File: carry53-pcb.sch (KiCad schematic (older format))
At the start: 127 parts, among them J1 Conn_01x02, J2 Conn_01x03, SW1 TS-1187A-B-A-B, SW2 TS-1187A-B-A-B, U1 STM32F072CBT6, U2 XC6206P332MR

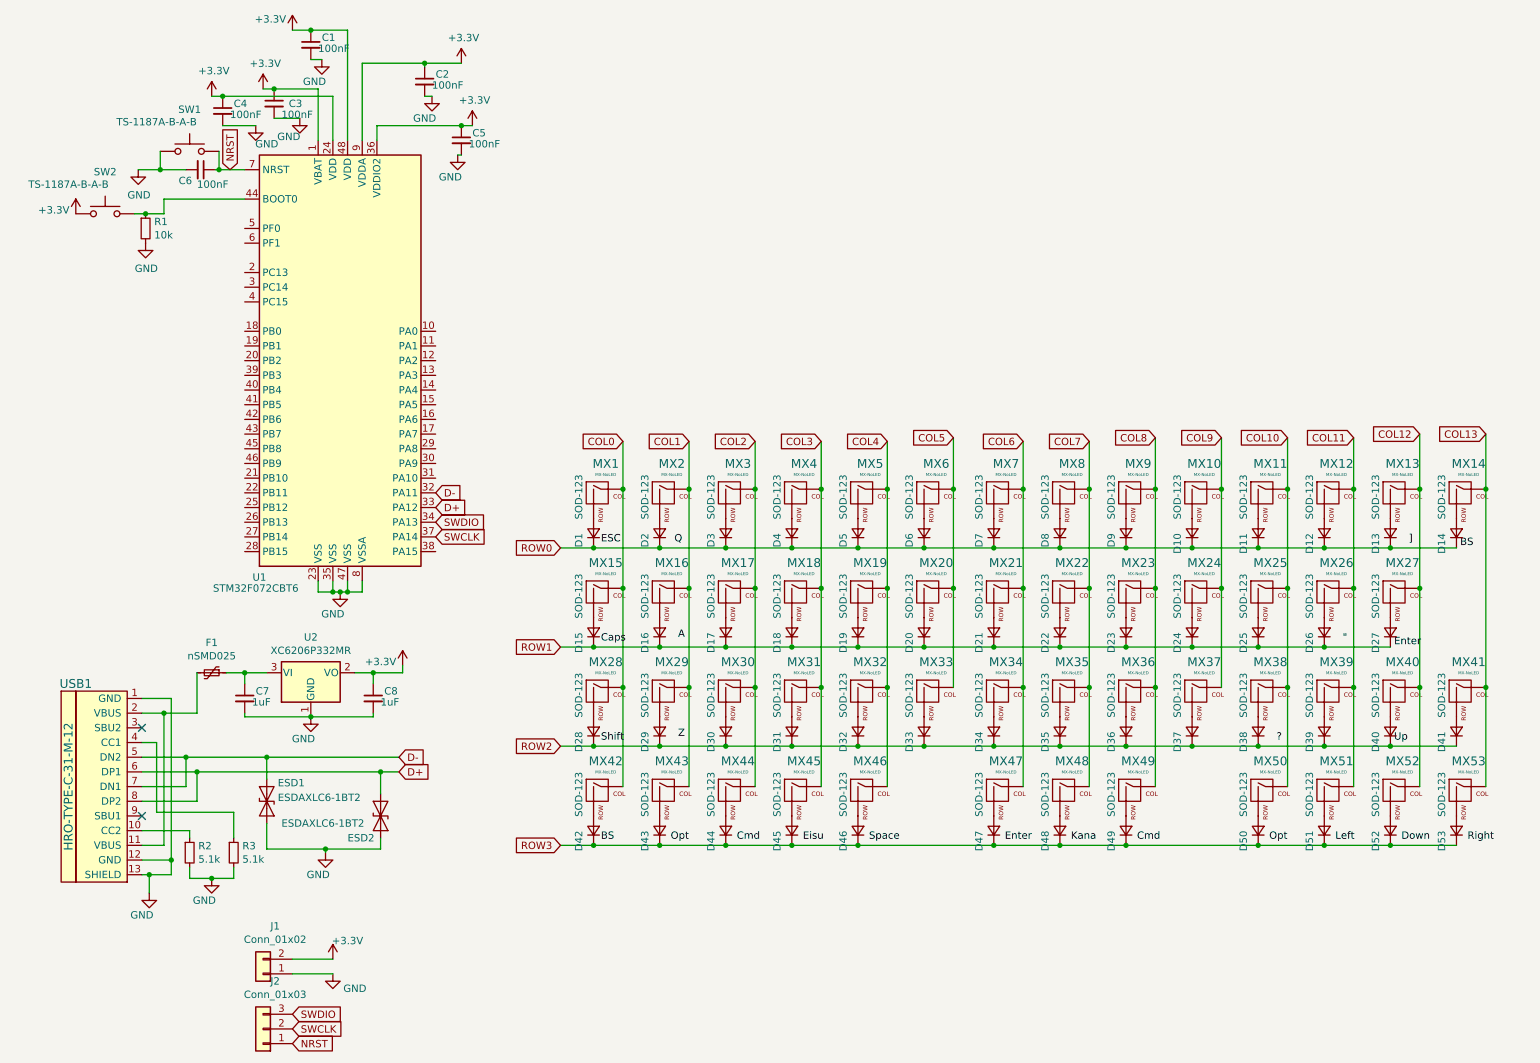
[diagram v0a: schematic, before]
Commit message: haisen_hobo_dekita
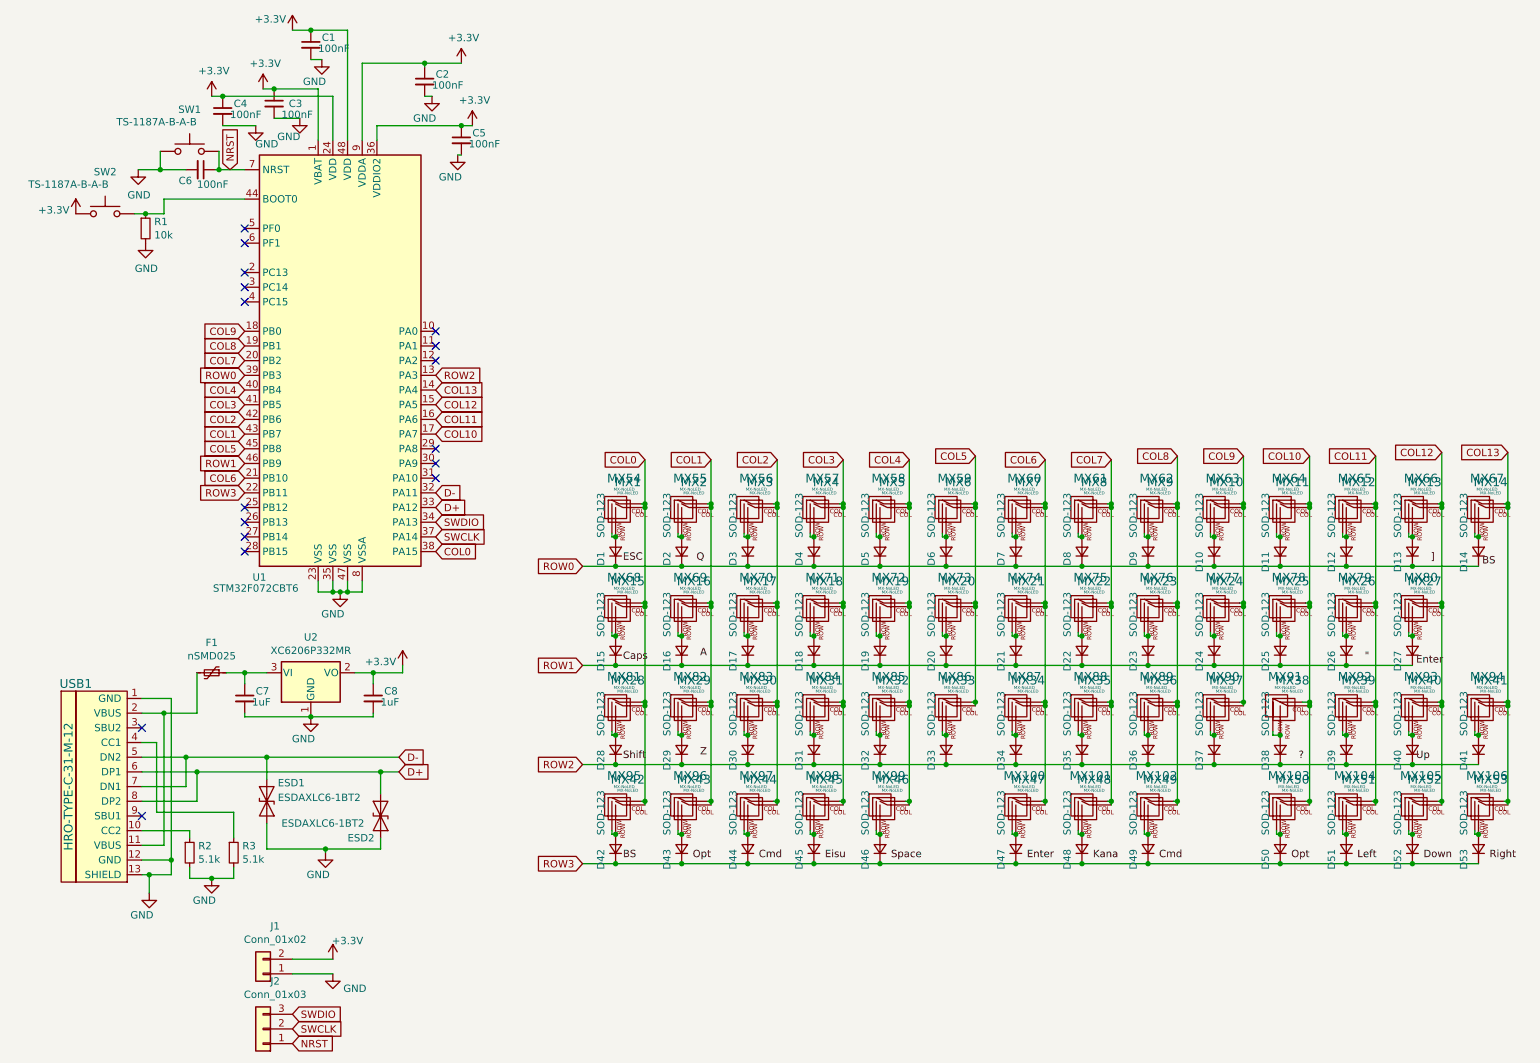
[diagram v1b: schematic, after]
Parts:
- added MX100, MX101, MX102, MX103, MX104, MX105, MX106, MX54, MX55, MX56, MX57, MX58, MX59, MX60, MX61, MX62, MX63, MX64, MX65, MX66, MX67, MX68, MX69, MX70, MX71, MX72, MX73, MX74, MX75, MX76, MX77, MX78, MX79, MX80, MX81, MX82, MX83, MX84, MX85, MX86, MX87, MX88, MX89, MX90, MX91, MX92, MX93, MX94, MX95, MX96, MX97, MX98, MX99: MX-NoLED, Kailh_Choc:KailhChoc-1U, symbol MX_Alps_Hybrid:MX-NoLED
- MX1, MX14, MX45, MX46, MX47: footprint (none) -> MX_Only:MXOnly-1.5U-NoLED
- MX10, MX11, MX12, MX13, MX16, MX17, MX18, MX19, MX2, MX20, MX21, MX22, MX23, MX24, MX25, MX26, MX29, MX3, MX30, MX31, MX32, MX33, MX34, MX35, MX36, MX37, MX38, MX39, MX4, MX40, MX41, MX5, MX51, MX52, MX53, MX6, MX7, MX8, MX9: footprint (none) -> MX_Only:MXOnly-1U-NoLED
- MX15: footprint (none) -> MX_Only:MXOnly-1.75U-NoLED
- MX27: footprint (none) -> MX_Only:MXOnly-2.25U-NoLED
- MX28: footprint (none) -> MX_Only:MXOnly-2U-NoLED
- MX42, MX43, MX44, MX48, MX49, MX50: footprint (none) -> MX_Only:MXOnly-1.25U-NoLED
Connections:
- net COL0: now also U1.38 (PA15), MX54.1 (COL), MX68.1 (COL), MX81.1 (COL), MX95.1 (COL)
- net COL1: now also U1.43 (PB7), MX55.1 (COL), MX69.1 (COL), MX82.1 (COL), MX96.1 (COL)
- net COL10: now also U1.17 (PA7), MX103.1 (COL), MX64.1 (COL), MX78.1 (COL), MX91.1 (COL)
- net COL11: now also U1.16 (PA6), MX104.1 (COL), MX65.1 (COL), MX79.1 (COL), MX92.1 (COL)
- net COL12: now also U1.15 (PA5), MX105.1 (COL), MX66.1 (COL), MX80.1 (COL), MX93.1 (COL)
- net COL13: now also U1.14 (PA4), MX106.1 (COL), MX67.1 (COL), MX94.1 (COL)
- net COL2: now also U1.42 (PB6), MX56.1 (COL), MX70.1 (COL), MX83.1 (COL), MX97.1 (COL)
- net COL3: now also U1.41 (PB5), MX57.1 (COL), MX71.1 (COL), MX84.1 (COL), MX98.1 (COL)
- net COL4: now also U1.40 (PB4), MX58.1 (COL), MX72.1 (COL), MX85.1 (COL), MX99.1 (COL)
- net COL5: now also U1.45 (PB8), MX59.1 (COL), MX73.1 (COL), MX86.1 (COL)
- net COL6: now also U1.21 (PB10), MX100.1 (COL), MX60.1 (COL), MX74.1 (COL), MX87.1 (COL)
- net COL7: now also U1.20 (PB2), MX101.1 (COL), MX61.1 (COL), MX75.1 (COL), MX88.1 (COL)
- net COL8: now also U1.19 (PB1), MX102.1 (COL), MX62.1 (COL), MX76.1 (COL), MX89.1 (COL)
- net COL9: now also U1.18 (PB0), MX63.1 (COL), MX77.1 (COL), MX90.1 (COL)
- net ROW0: now also U1.39 (PB3)
- net ROW1: now also U1.46 (PB9)
- net ROW2: now also U1.13 (PA3)
- net ROW3: now also U1.22 (PB11)
- net at D3.2 (A), MX3.2 (ROW): now also MX56.2 (ROW)
- net at D17.2 (A), MX17.2 (ROW): now also MX70.2 (ROW)
- net at D30.2 (A), MX30.2 (ROW): now also MX83.2 (ROW)
- net at D44.2 (A), MX44.2 (ROW): now also MX97.2 (ROW)
- net at D4.2 (A), MX4.2 (ROW): now also MX57.2 (ROW)
- net at D18.2 (A), MX18.2 (ROW): now also MX71.2 (ROW)
- net at D31.2 (A), MX31.2 (ROW): now also MX84.2 (ROW)
- net at D45.2 (A), MX45.2 (ROW): now also MX98.2 (ROW)
- net at D5.2 (A), MX5.2 (ROW): now also MX58.2 (ROW)
- net at D19.2 (A), MX19.2 (ROW): now also MX72.2 (ROW)
- net at D32.2 (A), MX32.2 (ROW): now also MX85.2 (ROW)
- net at D46.2 (A), MX46.2 (ROW): now also MX99.2 (ROW)
- net at D6.2 (A), MX6.2 (ROW): now also MX59.2 (ROW)
- net at D20.2 (A), MX20.2 (ROW): now also MX73.2 (ROW)
- net at D33.2 (A), MX33.2 (ROW): now also MX86.2 (ROW)
- net at D7.2 (A), MX7.2 (ROW): now also MX60.2 (ROW)
- net at D21.2 (A), MX21.2 (ROW): now also MX74.2 (ROW)
- net at D34.2 (A), MX34.2 (ROW): now also MX87.2 (ROW)
- net at D47.2 (A), MX47.2 (ROW): now also MX100.2 (ROW)
- net at D8.2 (A), MX8.2 (ROW): now also MX61.2 (ROW)
- net at D22.2 (A), MX22.2 (ROW): now also MX75.2 (ROW)
- net at D35.2 (A), MX35.2 (ROW): now also MX88.2 (ROW)
- net at D48.2 (A), MX48.2 (ROW): now also MX101.2 (ROW)
- net at D9.2 (A), MX9.2 (ROW): now also MX62.2 (ROW)
- net at D23.2 (A), MX23.2 (ROW): now also MX76.2 (ROW)
- net at D36.2 (A), MX36.2 (ROW): now also MX89.2 (ROW)
- net at D49.2 (A), MX49.2 (ROW): now also MX102.2 (ROW)
- net at D10.2 (A), MX10.2 (ROW): now also MX63.2 (ROW)
- net at D24.2 (A), MX24.2 (ROW): now also MX77.2 (ROW)
- net at D37.2 (A), MX37.2 (ROW): now also MX90.2 (ROW)
- net at D11.2 (A), MX11.2 (ROW): now also MX64.2 (ROW)
- net at D25.2 (A), MX25.2 (ROW): now also MX78.2 (ROW)
- net at D38.2 (A), MX38.2 (ROW): now also MX91.2 (ROW)
- net at D50.2 (A), MX50.2 (ROW): now also MX103.2 (ROW)
- net at D12.2 (A), MX12.2 (ROW): now also MX65.2 (ROW)
- net at D26.2 (A), MX26.2 (ROW): now also MX79.2 (ROW)
- net at D39.2 (A), MX39.2 (ROW): now also MX92.2 (ROW)
- net at D51.2 (A), MX51.2 (ROW): now also MX104.2 (ROW)
- net at D13.2 (A), MX13.2 (ROW): now also MX66.2 (ROW)
- net at D27.2 (A), MX27.2 (ROW): now also MX80.2 (ROW)
- net at D40.2 (A), MX40.2 (ROW): now also MX93.2 (ROW)
- net at D52.2 (A), MX52.2 (ROW): now also MX105.2 (ROW)
- net at D14.2 (A), MX14.2 (ROW): now also MX67.2 (ROW)
- net at D41.2 (A), MX41.2 (ROW): now also MX94.2 (ROW)
- net at D53.2 (A), MX53.2 (ROW): now also MX106.2 (ROW)
- net at D1.2 (A), MX1.2 (ROW): now also MX54.2 (ROW)
- net at D15.2 (A), MX15.2 (ROW): now also MX68.2 (ROW)
- net at D28.2 (A), MX28.2 (ROW): now also MX81.2 (ROW)
- net at D42.2 (A), MX42.2 (ROW): now also MX95.2 (ROW)
- net at D2.2 (A), MX2.2 (ROW): now also MX55.2 (ROW)
- net at D16.2 (A), MX16.2 (ROW): now also MX69.2 (ROW)
- net at D29.2 (A), MX29.2 (ROW): now also MX82.2 (ROW)
- net at D43.2 (A), MX43.2 (ROW): now also MX96.2 (ROW)
- no-connect marks 2 -> 17
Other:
- moved on the sheet: D1, D10, D11, D12, D13, D14, D15, D16, D17, D18, D19, D2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
